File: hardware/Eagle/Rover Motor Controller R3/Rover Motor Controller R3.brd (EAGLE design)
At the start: 12.7 x 25.4 mm, 9 parts

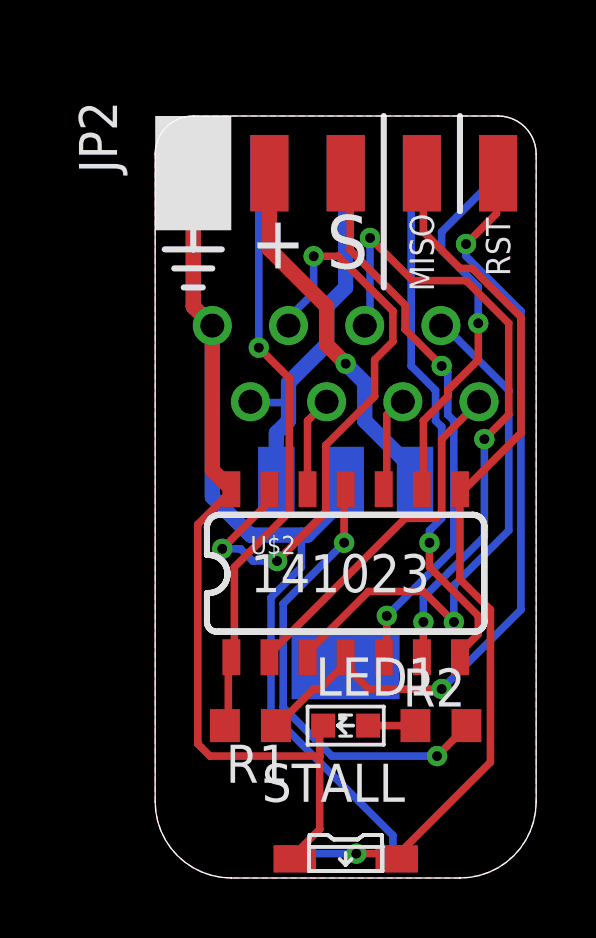
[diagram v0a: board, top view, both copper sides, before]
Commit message: Nothing to see here, move along
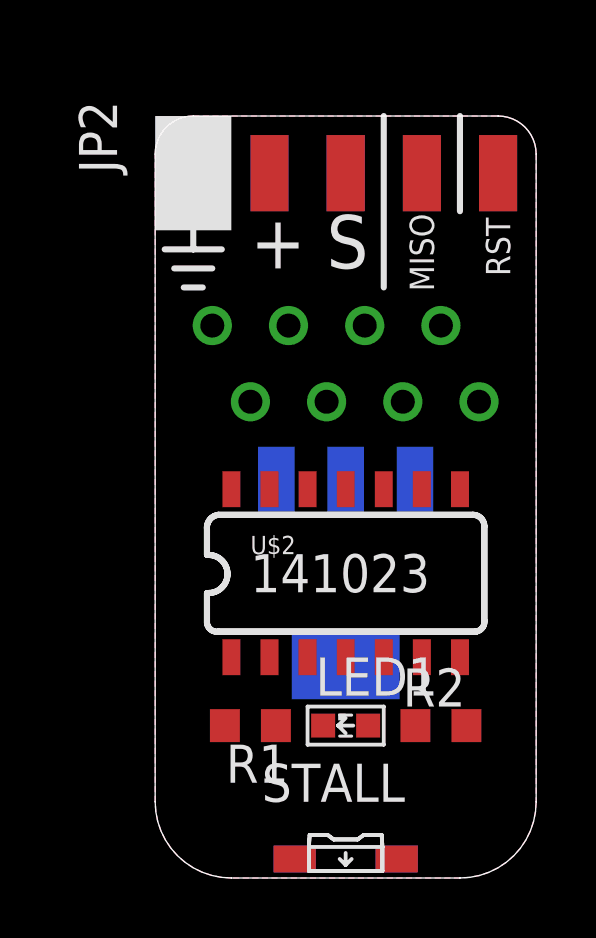
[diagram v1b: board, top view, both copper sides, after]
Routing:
- net GND: track 59.2 -> 0.00 mm
- net MISO: track 30.8 -> 0.00 mm, vias 1 -> 0
- net RST: track 26.9 -> 0.00 mm, vias 2 -> 0
- net PWM: track 21.1 -> 0.00 mm, vias 3 -> 0
- net IN1: track 20.8 -> 0.00 mm, vias 3 -> 0
- net +3V3: track 20.0 -> 0.00 mm, vias 1 -> 0
- net SERVO: track 18.6 -> 0.00 mm, vias 2 -> 0
- net QEA: track 18.0 -> 0.00 mm, vias 1 -> 0
- net SDA: track 17.8 -> 0.00 mm, vias 1 -> 0
- net STALL: track 15.5 -> 0.00 mm, vias 2 -> 0
- net SCL: track 12.6 -> 0.00 mm, vias 1 -> 0
- net VCC: track 12.5 -> 0.00 mm
- net +5V: track 12.2 -> 0.00 mm, vias 1 -> 0
- net QEB: track 12.0 -> 0.00 mm
- net STANDBY: track 3.25 -> 0.00 mm
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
